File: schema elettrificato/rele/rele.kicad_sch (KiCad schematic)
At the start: 8 parts, among them K1 Fujitsu_FTR-LYCA005x, K2 Fujitsu_FTR-LYCA005x, K3 Fujitsu_FTR-LYCA005x, K4 Fujitsu_FTR-LYCA005x, K5 Fujitsu_FTR-LYCA005x, K6 Fujitsu_FTR-LYCA005x, K7 Fujitsu_FTR-LYCA005x, K8 Fujitsu_FTR-LYCA005x

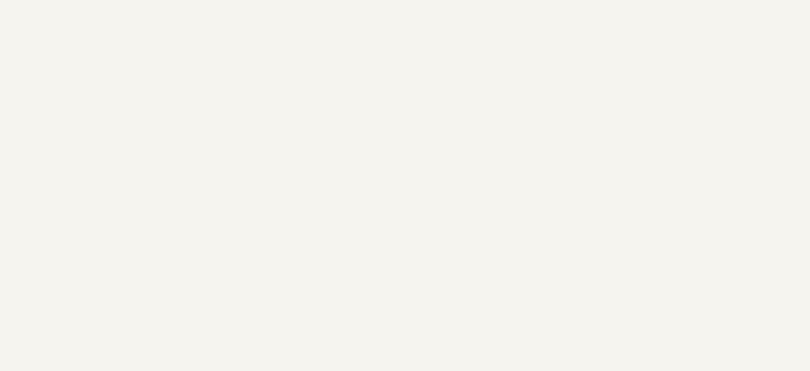
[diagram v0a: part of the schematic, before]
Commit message: a
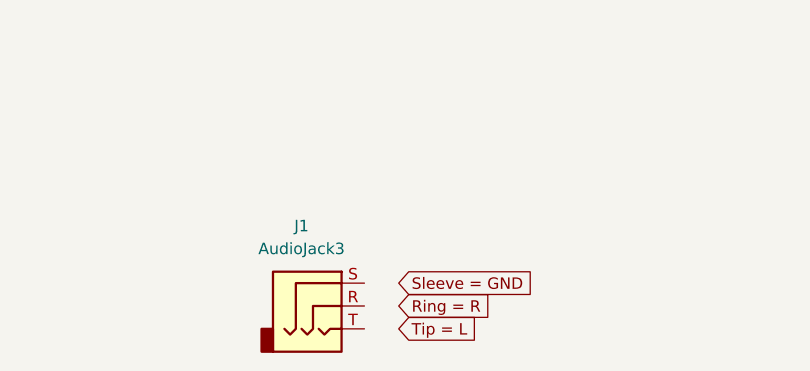
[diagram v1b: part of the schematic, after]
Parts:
- added J1: AudioJack3, symbol Connector_Audio:AudioJack3
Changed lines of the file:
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@@
+		)
+	)
+	(global_label "Ring = R"
+		(shape input)
+		(at 66.04 120.65 0)
+		(fields_autoplaced yes)
+		(effects
+			(font
+				(size 1.27 1.27)
+			)
+			(justify left)
+		)
+		(property "Intersheetrefs" "${INTERSHEET_REFS}"
+			(at 77.9756 120.65 0)
+			(effects
+				(font
+					(size 1.27 1.27)
+				)
+				(justify left)
+				(hide yes)
+			)
 		)
 	)
@@
 		)
 	)
+	(global_label "Tip = L"
+		(shape input)
+		(at 66.04 123.19 0)
+		(fields_autoplaced yes)
+		(effects
+			(font
+				(size 1.27 1.27)
+			)
+			(justify left)
+		)
+		(property "Intersheetrefs" "${INTERSHEET_REFS}"
+			(at 76.2823 123.19 0)
+			(effects
+				(font
+					(size 1.27 1.27)
+				)
+				(justify left)
+				(hide yes)
+			)
+		)
+	)
 	(global_label "Out 4"
 		(shape input)
@@
 		(property "Intersheetrefs" "${INTERSHEET_REFS}"
 			(at 129.54 25.9225 90)
+			(effects
+				(font
+					(size 1.27 1.27)
+				)
+				(justify left)
+				(hide yes)
+			)
+		)
+	)
+	(global_label "Sleeve = GND"
+		(shape input)
+		(at 66.04 118.11 0)
+		(fields_autoplaced yes)
+		(effects
+			(font
+				(size 1.27 1.27)
+			)
+			(justify left)
+		)
+		(property "Intersheetrefs" "${INTERSHEET_REFS}"
+			(at 82.5114 118.11 0)
 			(effects
 				(font
@@
 					(unit 1)
 				)
+			)
+		)
+	)
+	(symbol
+		(lib_id "Connector_Audio:AudioJack3")
+		(at 57.15 120.65 0)
+		(unit 1)
+		(exclude_from_sim no)
+		(in_bom yes)
+		(on_board yes)
+		(dnp no)
+		(fields_autoplaced yes)
+		(property "Reference" "J1"
+			(at 55.245 111.76 0)
+			(effects
+				(font
+					(size 1.27 1.27)
+				)
+			)
+		)
+		(property "Value" "AudioJack3"
+			(at 55.245 114.3 0)
+			(effects
+				(font
+					(size 1.27 1.27)
+				)
+			)
+		)
+		(property "Footprint" ""
+			(at 57.15 120.65 0)
+			(effects
+				(font
+					(size 1.27 1.27)
+				)
+				(hide yes)
+			)
+		)
+		(property "Datasheet" "~"
+			(at 57.15 120.65 0)
+			(effects
+				(font
+					(size 1.27 1.27)
+				)
+				(hide yes)
+			)
+		)
+		(property "Description" "Audio Jack, 3 Poles (Stereo / TRS)"
+			(at 57.15 120.65 0)
+			(effects
+				(font
+					(size 1.27 1.27)
+				)
+				(hide yes)
+			)
+		)
+		(pin "S"
+		)
+		(pin "R"
+		)
+		(pin "T"
+		)
+		(instances
+			(project ""
+				(path "/604ae42d-a464-4564-8245-f9eef8e99996"
+					(reference "J1")
+					(unit 1)
+				)
